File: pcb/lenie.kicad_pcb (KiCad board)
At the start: 2 copper layers, 3 parts, among them J1 Conn_01x05_MountingPin, U1 CR2013-MI2120, U2 ESP32-DEVKIT-V1

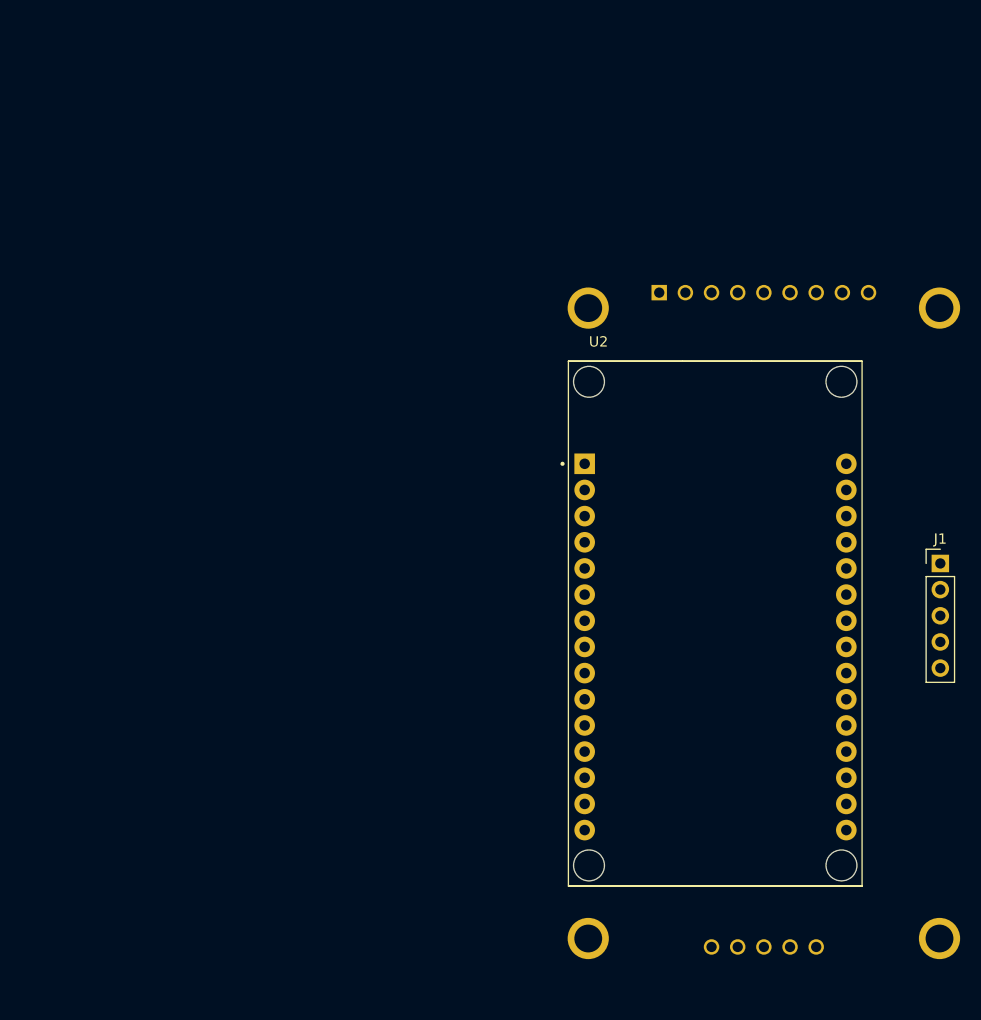
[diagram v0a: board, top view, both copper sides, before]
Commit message: vault backup: 2025-06-01 16:34:12
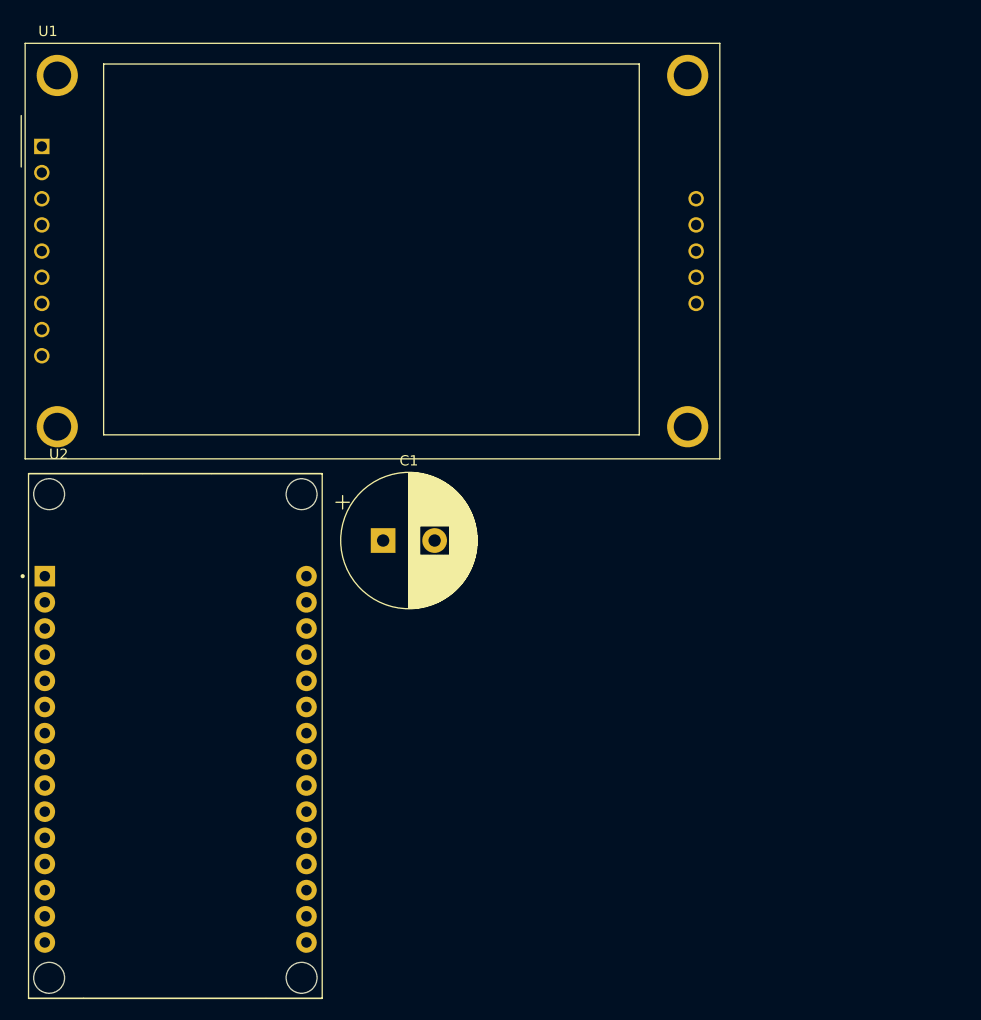
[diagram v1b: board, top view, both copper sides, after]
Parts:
- removed J1: Conn_01x05_MountingPin, Connector_PinHeader_2.54mm:PinHeader_1x05_P2.54mm_Vertical
- added C1: 2200uF 25V, PCM_Capacitor_THT_AKL:CP_Radial_D13.0mm_P5.00mm, F.Cu at (101.6, 100.7)
- U1: moved to F.Cu
- moved U1 61.6 mm to (68.5, 62.4), turned to 0 degrees
- moved U2 53.5 mm to (81.5, 119.6)
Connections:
- net GND renamed -BATT
- U1 pad 14: +3V3 -> SD_DETECT
- U2 pad 10: MISO -> TFT_LED
- U2 pad 11: unconnected-(U2-D21-Pad11) -> DS3231_SDA
- U2 pad 14: TFT_LED -> DS3231_SCL
- U2 pad 15: unconnected-(U2-D23-Pad15) -> Button_1
- U2 pad 16: unconnected-(U2-EN-Pad16) -> ESP32_EN
- U2 pad 17: unconnected-(U2-VP-Pad17) -> BATTERY_LEVEL
- U2 pad 19: unconnected-(U2-D34-Pad19) -> SD_DETECT
- U2 pad 23: MOSI -> PAM8403_L
- U2 pad 24: Button_1 -> PAM8403_R
- U2 pad 26: LED_SCK -> SCK
- U2 pad 27: unconnected-(U2-D12-Pad27) -> MISO
- U2 pad 28: LED_DIN -> MOSI
- U2 pad 3: SD_CS -> TFT_CS
- U2 pad 5: unconnected-(U2-D4-Pad5) -> TFT_RST
- U2 pad 8: TFT_CS -> SD_CS
- U2 pad 9: SCK -> LED_SCK
